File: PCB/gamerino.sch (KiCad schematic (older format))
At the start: 47 parts, among them J1 USB_B_Micro, J2 LT2, J3 RT2, P1 JOY1, P2 JOY2, P3 ICSP, P4 AUX, SW1 HATSWITCH, SW10 OPTS, SW11 X, SW12 B, SW13 A, SW14 Y, SW2 LT1, SW3 LT2, SW4 RT1, SW5 RT2, SW6 SEL, SW7 START, SW8 CLEAR, SW9 HOME, U1 MIC5219-3.3YM5, U2 ATmega32U4, U3 TCA6416A, X1 16MHz

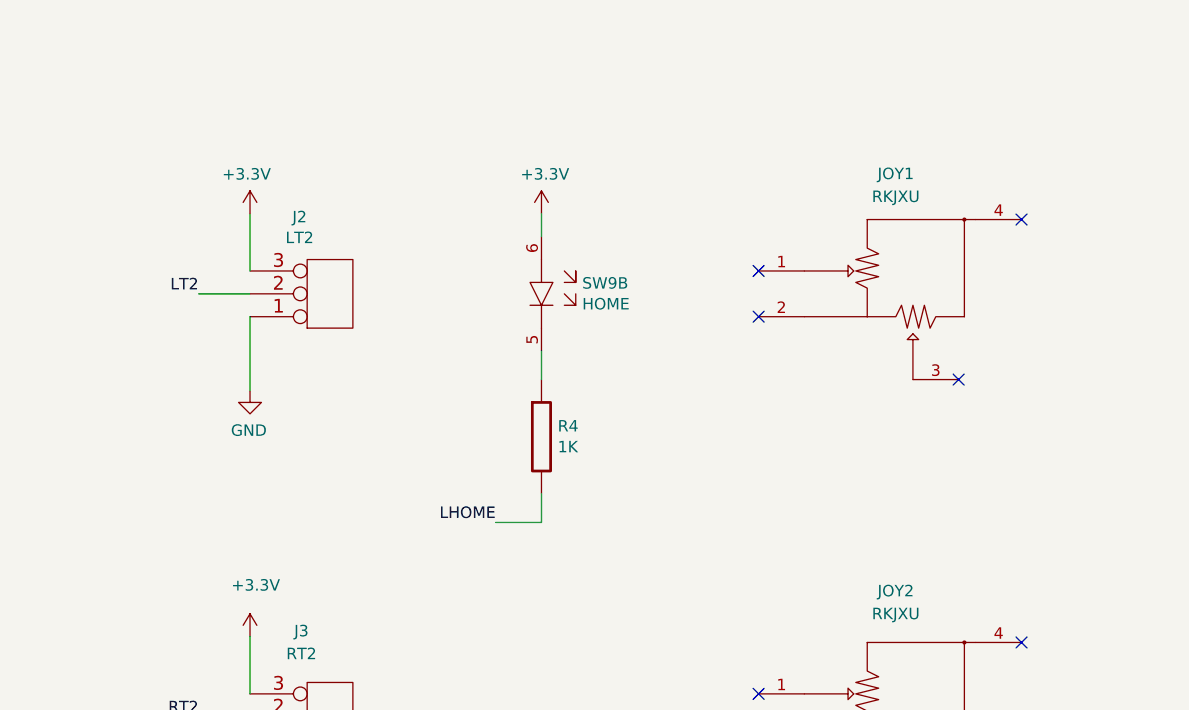
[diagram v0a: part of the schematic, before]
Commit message: Update
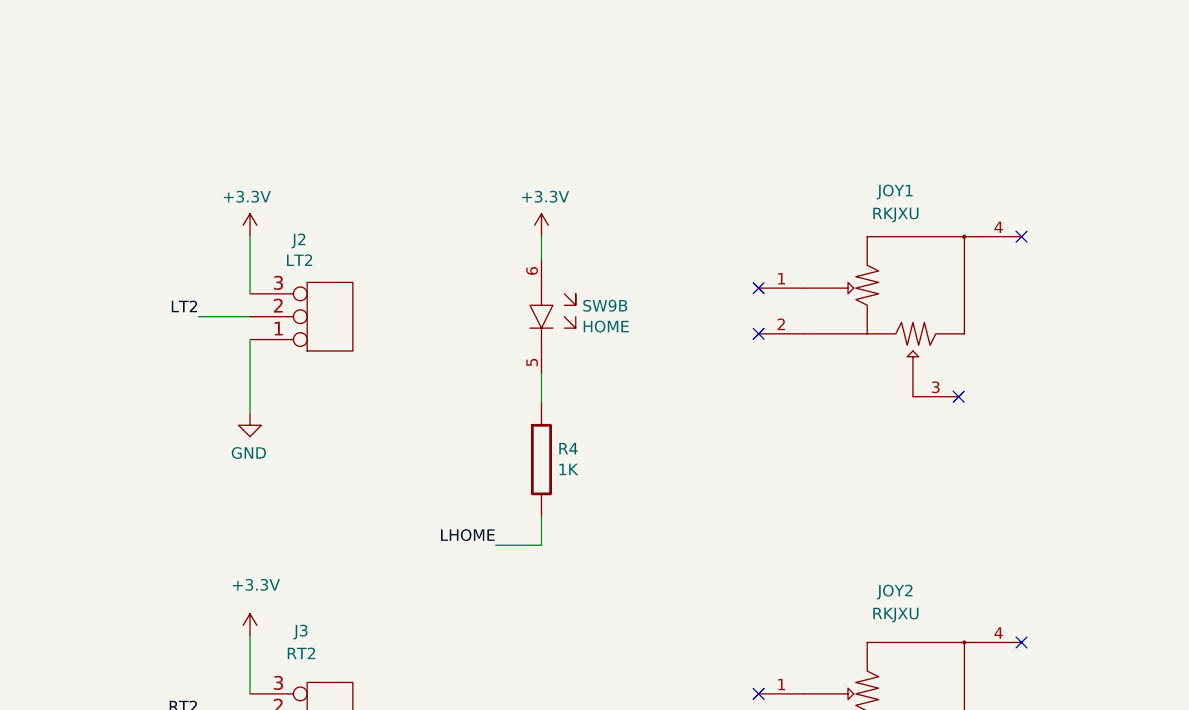
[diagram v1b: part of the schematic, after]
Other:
- moved on the sheet: J2, JOY1, R4, SW9B
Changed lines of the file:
@@
 	7825 9925 7600 9925
 Wire Wire Line
-	7600 8075 7825 8075
+	7600 8175 7825 8175
 $Comp
 L gamerino-rescue:GND-power #PWR026
@@
 L gamerino-rescue:R-device R4
 U 1 1 60E4EB67
-P 9100 8700
-F 0 "R4" H 9171 8746 50  0000 L CNN
-F 1 "1K" H 9171 8655 50  0000 L CNN
-F 2 "Resistor_SMD:R_0603_1608Metric" V 9030 8700 30  0001 C CNN
-F 3 "" H 9100 8700 30  0000 C CNN
-F 4 "CRG0603F1K0" H 9100 8700 50  0001 C CNN "MPN"
-F 5 "TE" H 9100 8700 50  0001 C CNN "Manufacturer"
-F 6 "A106049CT-ND" H 9100 8700 50  0001 C CNN "Digikey"
-F 7 "279-CRG0603F1K0" H 9100 8700 50  0001 C CNN "Mouser"
-F 8 "213-2266" H 9100 8700 50  0001 C CNN "RS"
-F 9 "3399571" H 9100 8700 50  0001 C CNN "Farnell"
-	1    9100 8700
+P 9100 8800
+F 0 "R4" H 9171 8846 50  0000 L CNN
+F 1 "1K" H 9171 8755 50  0000 L CNN
+F 2 "Resistor_SMD:R_0603_1608Metric" V 9030 8800 30  0001 C CNN
+F 3 "" H 9100 8800 30  0000 C CNN
+F 4 "CRG0603F1K0" H 9100 8800 50  0001 C CNN "MPN"
+F 5 "TE" H 9100 8800 50  0001 C CNN "Manufacturer"
+F 6 "A106049CT-ND" H 9100 8800 50  0001 C CNN "Digikey"
+F 7 "279-CRG0603F1K0" H 9100 8800 50  0001 C CNN "Mouser"
+F 8 "213-2266" H 9100 8800 50  0001 C CNN "RS"
+F 9 "3399571" H 9100 8800 50  0001 C CNN "Farnell"
+	1    9100 8800
 	1    0    0    -1
 $EndComp
@@
 Text Label 10500 4950 0    50   ~ 0
 RT1
-Text Label 7600 8075 2    50   ~ 0
+Text Label 7600 8175 2    50   ~ 0
 LT2
 Text Label 7600 9925 2    50   ~ 0
@@
 L gamerino-rescue:+3.3V-power #PWR023
 U 1 1 6116AC53
-P 7825 7725
-F 0 "#PWR023" H 7825 7575 50  0001 C CNN
-F 1 "+3.3V" H 7840 7898 50  0000 C CNN
-F 2 "" H 7825 7725 50  0001 C CNN
-F 3 "" H 7825 7725 50  0001 C CNN
-	1    7825 7725
+P 7825 7825
+F 0 "#PWR023" H 7825 7675 50  0001 C CNN
+F 1 "+3.3V" H 7840 7998 50  0000 C CNN
+F 2 "" H 7825 7825 50  0001 C CNN
+F 3 "" H 7825 7825 50  0001 C CNN
+	1    7825 7825
 	-1   0    0    -1
 $EndComp
@@
 L gamerino-rescue:GND-power #PWR024
 U 1 1 6116B2BE
-P 7825 8500
-F 0 "#PWR024" H 7825 8250 50  0001 C CNN
-F 1 "GND" H 7830 8327 50  0000 C CNN
-F 2 "" H 7825 8500 50  0001 C CNN
-F 3 "" H 7825 8500 50  0001 C CNN
-	1    7825 8500
+P 7825 8600
+F 0 "#PWR024" H 7825 8350 50  0001 C CNN
+F 1 "GND" H 7830 8427 50  0000 C CNN
+F 2 "" H 7825 8600 50  0001 C CNN
+F 3 "" H 7825 8600 50  0001 C CNN
+	1    7825 8600
 	-1   0    0    -1
 $EndComp
 Wire Wire Line
-	7825 7725 7825 7975
-Wire Wire Line
-	7825 8175 7825 8500
+	7825 7825 7825 8075
+Wire Wire Line
+	7825 8275 7825 8600
 $Comp
 L gamerino-rescue:CONN_3-conn J2
 U 1 1 6116B2CB
-P 8175 8075
-F 0 "J2" H 8042 7739 50  0000 C CNN
-F 1 "LT2" H 8042 7830 50  0000 C CNN
-F 2 "gamerino:Molex_PicoBlade_53047-0310_1x03_P1.25mm_Vertical" H 8175 8075 50  0001 C CNN
-F 3 "" H 8175 8075 50  0001 C CNN
-F 4 "53047-0310" H 8175 8075 50  0001 C CNN "MPN"
-F 5 "Molex" H 8175 8075 50  0001 C CNN "Manufacturer"
-F 6 "WM1732-ND" H 8175 8075 50  0001 C CNN "Digikey"
-F 7 "538-53047-0310" H 8175 8075 50  0001 C CNN "Mouser"
-F 8 "319-1064" H 8175 8075 50  0001 C CNN "RS"
-F 9 "9732853" H 8175 8075 50  0001 C CNN "Farnell"
-	1    8175 8075
+P 8175 8175
+F 0 "J2" H 8042 7839 50  0000 C CNN
+F 1 "LT2" H 8042 7930 50  0000 C CNN
+F 2 "gamerino:Molex_PicoBlade_53047-0310_1x03_P1.25mm_Vertical" H 8175 8175 50  0001 C CNN
+F 3 "" H 8175 8175 50  0001 C CNN
+F 4 "53047-0310" H 8175 8175 50  0001 C CNN "MPN"
+F 5 "Molex" H 8175 8175 50  0001 C CNN "Manufacturer"
+F 6 "WM1732-ND" H 8175 8175 50  0001 C CNN "Digikey"
+F 7 "538-53047-0310" H 8175 8175 50  0001 C CNN "Mouser"
+F 8 "319-1064" H 8175 8175 50  0001 C CNN "RS"
+F 9 "9732853" H 8175 8175 50  0001 C CNN "Farnell"
+	1    8175 8175
 	1    0    0    1
 $EndComp
@@
 Connection ~ 14900 2950
 Wire Wire Line
-	9100 8450 9100 8325
-Wire Wire Line
-	9100 8950 9100 9075
+	9100 8550 9100 8425
+Wire Wire Line
+	9100 9050 9100 9175
 $Comp
 L gamerino-rescue:+3.3V-power #PWR0103
 U 1 1 60C0ACCD
-P 9100 7725
-F 0 "#PWR0103" H 9100 7575 50  0001 C CNN
-F 1 "+3.3V" H 9115 7898 50  0000 C CNN
-F 2 "" H 9100 7725 50  0001 C CNN
-F 3 "" H 9100 7725 50  0001 C CNN
-	1    9100 7725
+P 9100 7825
+F 0 "#PWR0103" H 9100 7675 50  0001 C CNN
+F 1 "+3.3V" H 9115 7998 50  0000 C CNN
+F 2 "" H 9100 7825 50  0001 C CNN
+F 3 "" H 9100 7825 50  0001 C CNN
+	1    9100 7825
 	1    0    0    -1
 $EndComp
@@
 L gamerino:TL1 SW9
 U 2 1 60C5CD0F
-P 8800 8075
-F 0 "SW9" V 8846 7597 50  0000 R CNN
-F 1 "HOME" V 8755 7597 50  0000 R CNN
-F 2 "gamerino:TL3265" H 8800 8225 50  0001 C CNN
-F 3 "" H 8800 8225 50  0001 C CNN
-F 4 "TL3265GQSCLR" H 8800 8075 50  0001 C CNN "MPN"
-F 5 "E-Switch" H 8800 8075 50  0001 C CNN "Manufacturer"
-F 6 "EG5518CT-ND" H 8800 8075 50  0001 C CNN "Digikey"
-F 7 "612-TL3265GQSCLR" H 8800 8075 50  0001 C CNN "Mouser"
-	2    8800 8075
+P 8800 8175
+F 0 "SW9" V 8846 7697 50  0000 R CNN
+F 1 "HOME" V 8755 7697 50  0000 R CNN
+F 2 "gamerino:TL3265" H 8800 8325 50  0001 C CNN
+F 3 "" H 8800 8325 50  0001 C CNN
+F 4 "TL3265GQSCLR" H 8800 8175 50  0001 C CNN "MPN"
+F 5 "E-Switch" H 8800 8175 50  0001 C CNN "Manufacturer"
+F 6 "EG5518CT-ND" H 8800 8175 50  0001 C CNN "Digikey"
+F 7 "612-TL3265GQSCLR" H 8800 8175 50  0001 C CNN "Mouser"
+	2    8800 8175
 	0    -1   -1   0
 $EndComp
 Wire Wire Line
-	9100 7825 9100 7725
+	9100 7925 9100 7825
 Wire Wire Line
 	14725 4325 14900 4325
@@
 L gamerino:RKJXU JOY1
 U 1 1 60AED526
-P 10725 7975
-F 0 "JOY1" H 10650 8400 50  0000 C CNN
-F 1 "RKJXU" H 10650 8300 50  0000 C CNN
-F 2 "gamerino:RKJXU" H 10050 7975 50  0001 C CNN
-F 3 "" H 10050 7975 50  0001 C CNN
-F 4 "RKJXU1210006" H 10725 7975 50  0001 C CNN "MPN"
-F 5 "ALPS Alpine" H 10725 7975 50  0001 C CNN "Manufacturer"
-F 6 "688-RKJXU1210006" H 10725 7975 50  0001 C CNN "Mouser"
-	1    10725 7975
+P 10725 8050
+F 0 "JOY1" H 10650 8475 50  0000 C CNN
+F 1 "RKJXU" H 10650 8375 50  0000 C CNN
+F 2 "gamerino:RKJXU" H 10050 8050 50  0001 C CNN
+F 3 "" H 10050 8050 50  0001 C CNN
+F 4 "RKJXU1210006" H 10725 8050 50  0001 C CNN "MPN"
+F 5 "ALPS Alpine" H 10725 8050 50  0001 C CNN "Manufacturer"
+F 6 "688-RKJXU1210006" H 10725 8050 50  0001 C CNN "Mouser"
+	1    10725 8050
 	1    0    0    -1
 $EndComp
@@
 NoConn ~ 10925 10300
 NoConn ~ 11200 9600
-NoConn ~ 11200 7750
-NoConn ~ 10050 7975
-NoConn ~ 10050 8175
-NoConn ~ 10925 8450
-Wire Wire Line
-	9100 9075 8900 9075
-Text Label 8900 9075 2    50   ~ 0
+NoConn ~ 11200 7825
+NoConn ~ 10050 8050
+NoConn ~ 10050 8250
+NoConn ~ 10925 8525
+Wire Wire Line
+	9100 9175 8900 9175
+Text Label 8900 9175 2    50   ~ 0
 LHOME
 Text Label 4725 4550 0    50   ~ 0
